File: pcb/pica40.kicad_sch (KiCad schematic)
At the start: 65 parts, among them SW1 SW_PUSH, SW10 SW_PUSH, SW11 SW_PUSH, SW12 SW_PUSH, SW13 SW_PUSH, SW14 SW_PUSH, SW15 SW_PUSH, SW16 SW_PUSH, SW17 SW_PUSH, SW18 SW_PUSH, SW19 SW_PUSH, SW2 SW_PUSH, SW20 SW_PUSH, SW3 SW_PUSH, SW4 SW_PUSH, SW5 SW_PUSH, SW6 SW_PUSH, SW7 SW_PUSH, SW8 SW_PUSH, SW9 SW_PUSH, U1 ProMicro

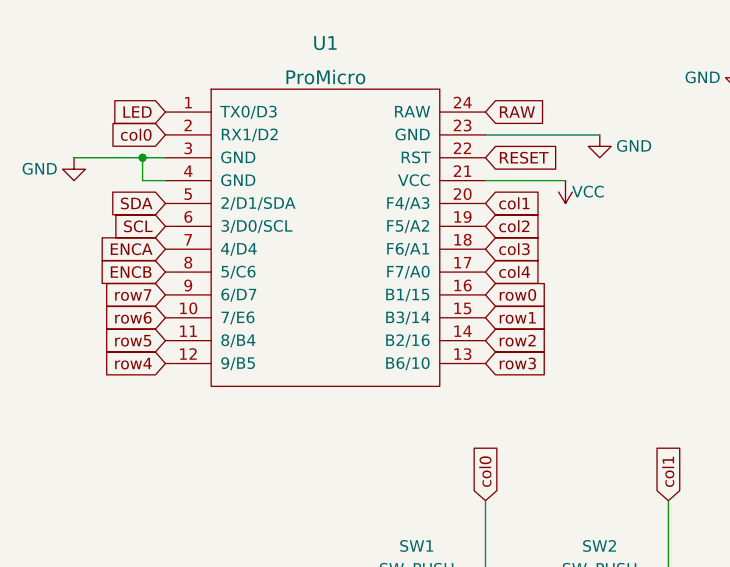
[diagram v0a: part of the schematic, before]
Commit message: update and reroute
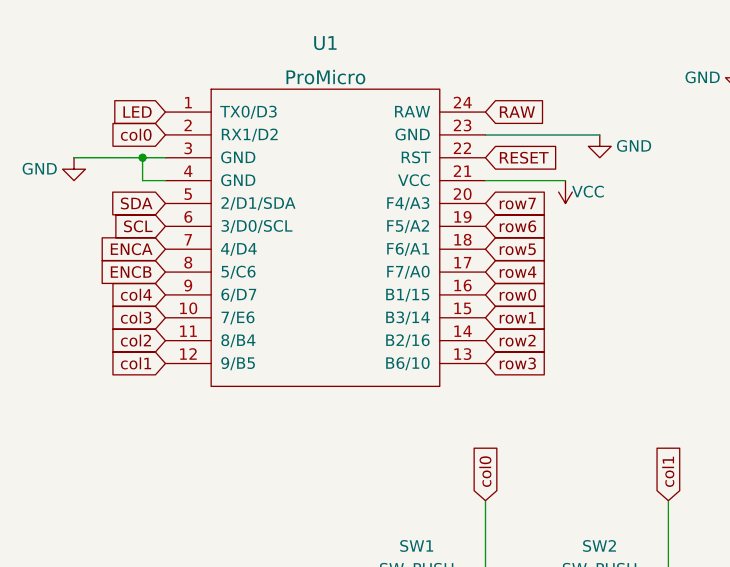
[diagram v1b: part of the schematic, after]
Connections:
- net col1: now also U1.12 (9/B5); no longer U1.20 (F4/A3)
- net col2: now also U1.11 (8/B4); no longer U1.19 (F5/A2)
- net col3: now also U1.10 (7/E6); no longer U1.18 (F6/A1)
- net col4: now also U1.9 (6/D7); no longer U1.17 (F7/A0)
- net row4: now also U1.17 (F7/A0); no longer U1.12 (9/B5)
- net row5: now also U1.18 (F6/A1); no longer U1.11 (8/B4)
- net row6: now also U1.19 (F5/A2); no longer U1.10 (7/E6)
- net row7: now also U1.20 (F4/A3); no longer U1.9 (6/D7)
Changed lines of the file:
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@@
     )
   )
-  (global_label "col1" (shape input) (at 69.85 45.72 0) (fields_autoplaced)
-    (effects (font (size 1.27 1.27)) (justify left))
-    (property "Intersheet References" "${INTERSHEET_REFS}" (id 0) (at 76.3755 45.7994 0)
-      (effects (font (size 1.27 1.27)) (justify left) hide)
+  (global_label "col1" (shape input) (at 34.29 63.5 180) (fields_autoplaced)
+    (effects (font (size 1.27 1.27)) (justify right))
+    (property "Intersheet References" "${INTERSHEET_REFS}" (id 0) (at 27.7645 63.4206 0)
+      (effects (font (size 1.27 1.27)) (justify right) hide)
     )
   )
@@
     )
   )
-  (global_label "col4" (shape input) (at 69.85 53.34 0) (fields_autoplaced)
-    (effects (font (size 1.27 1.27)) (justify left))
-    (property "Intersheet References" "${INTERSHEET_REFS}" (id 0) (at 76.3755 53.4194 0)
-      (effects (font (size 1.27 1.27)) (justify left) hide)
-    )
-  )
-  (global_label "row5" (shape input) (at 34.29 60.96 180) (fields_autoplaced)
-    (effects (font (size 1.27 1.27)) (justify right))
-    (property "Intersheet References" "${INTERSHEET_REFS}" (id 0) (at 27.4017 61.0394 0)
-      (effects (font (size 1.27 1.27)) (justify right) hide)
+  (global_label "col4" (shape input) (at 34.29 55.88 180) (fields_autoplaced)
+    (effects (font (size 1.27 1.27)) (justify right))
+    (property "Intersheet References" "${INTERSHEET_REFS}" (id 0) (at 27.7645 55.8006 0)
+      (effects (font (size 1.27 1.27)) (justify right) hide)
+    )
+  )
+  (global_label "row5" (shape input) (at 69.85 50.8 0) (fields_autoplaced)
+    (effects (font (size 1.27 1.27)) (justify left))
+    (property "Intersheet References" "${INTERSHEET_REFS}" (id 0) (at 76.7383 50.7206 0)
+      (effects (font (size 1.27 1.27)) (justify left) hide)
     )
   )
@@
     )
   )
-  (global_label "col2" (shape input) (at 69.85 48.26 0) (fields_autoplaced)
-    (effects (font (size 1.27 1.27)) (justify left))
-    (property "Intersheet References" "${INTERSHEET_REFS}" (id 0) (at 76.3755 48.3394 0)
-      (effects (font (size 1.27 1.27)) (justify left) hide)
+  (global_label "col2" (shape input) (at 34.29 60.96 180) (fields_autoplaced)
+    (effects (font (size 1.27 1.27)) (justify right))
+    (property "Intersheet References" "${INTERSHEET_REFS}" (id 0) (at 27.7645 60.8806 0)
+      (effects (font (size 1.27 1.27)) (justify right) hide)
     )
   )
@@
     )
   )
-  (global_label "row6" (shape input) (at 34.29 58.42 180) (fields_autoplaced)
-    (effects (font (size 1.27 1.27)) (justify right))
-    (property "Intersheet References" "${INTERSHEET_REFS}" (id 0) (at 27.4017 58.4994 0)
-      (effects (font (size 1.27 1.27)) (justify right) hide)
+  (global_label "row6" (shape input) (at 69.85 48.26 0) (fields_autoplaced)
+    (effects (font (size 1.27 1.27)) (justify left))
+    (property "Intersheet References" "${INTERSHEET_REFS}" (id 0) (at 76.7383 48.1806 0)
+      (effects (font (size 1.27 1.27)) (justify left) hide)
     )
   )
@@
     )
   )
-  (global_label "col3" (shape input) (at 69.85 50.8 0) (fields_autoplaced)
-    (effects (font (size 1.27 1.27)) (justify left))
-    (property "Intersheet References" "${INTERSHEET_REFS}" (id 0) (at 76.3755 50.8794 0)
-      (effects (font (size 1.27 1.27)) (justify left) hide)
+  (global_label "col3" (shape input) (at 34.29 58.42 180) (fields_autoplaced)
+    (effects (font (size 1.27 1.27)) (justify right))
+    (property "Intersheet References" "${INTERSHEET_REFS}" (id 0) (at 27.7645 58.3406 0)
+      (effects (font (size 1.27 1.27)) (justify right) hide)
     )
   )
@@
     )
   )
-  (global_label "row4" (shape input) (at 34.29 63.5 180) (fields_autoplaced)
-    (effects (font (size 1.27 1.27)) (justify right))
-    (property "Intersheet References" "${INTERSHEET_REFS}" (id 0) (at 27.4017 63.5794 0)
-      (effects (font (size 1.27 1.27)) (justify right) hide)
+  (global_label "row4" (shape input) (at 69.85 53.34 0) (fields_autoplaced)
+    (effects (font (size 1.27 1.27)) (justify left))
+    (property "Intersheet References" "${INTERSHEET_REFS}" (id 0) (at 76.7383 53.2606 0)
+      (effects (font (size 1.27 1.27)) (justify left) hide)
     )
   )
@@
     )
   )
-  (global_label "row7" (shape input) (at 34.29 55.88 180) (fields_autoplaced)
-    (effects (font (size 1.27 1.27)) (justify right))
-    (property "Intersheet References" "${INTERSHEET_REFS}" (id 0) (at 27.4017 55.9594 0)
-      (effects (font (size 1.27 1.27)) (justify right) hide)
-    )
-  )
+  (global_label "row7" (shape input) (at 69.85 45.72 0) (fields_autoplaced)
+    (effects (font (size 1.27 1.27)) (justify left))
+    (property "Intersheet References" "${INTERSHEET_REFS}" (id 0) (at 76.7383 45.6406 0)
+      (effects (font (size 1.27 1.27)) (justify left) hide)
+    )
+  )
